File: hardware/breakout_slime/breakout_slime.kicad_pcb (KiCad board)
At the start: 2 copper layers, 54.6 x 35.6 mm, 11 parts, among them J1 Battery_Connector, J2 IMU_Conn_Female, SW1 SW_SPDT, U1 TP4056_Breakout, U2 WeMos_D1_mini, U3 BNO/MPU_Break

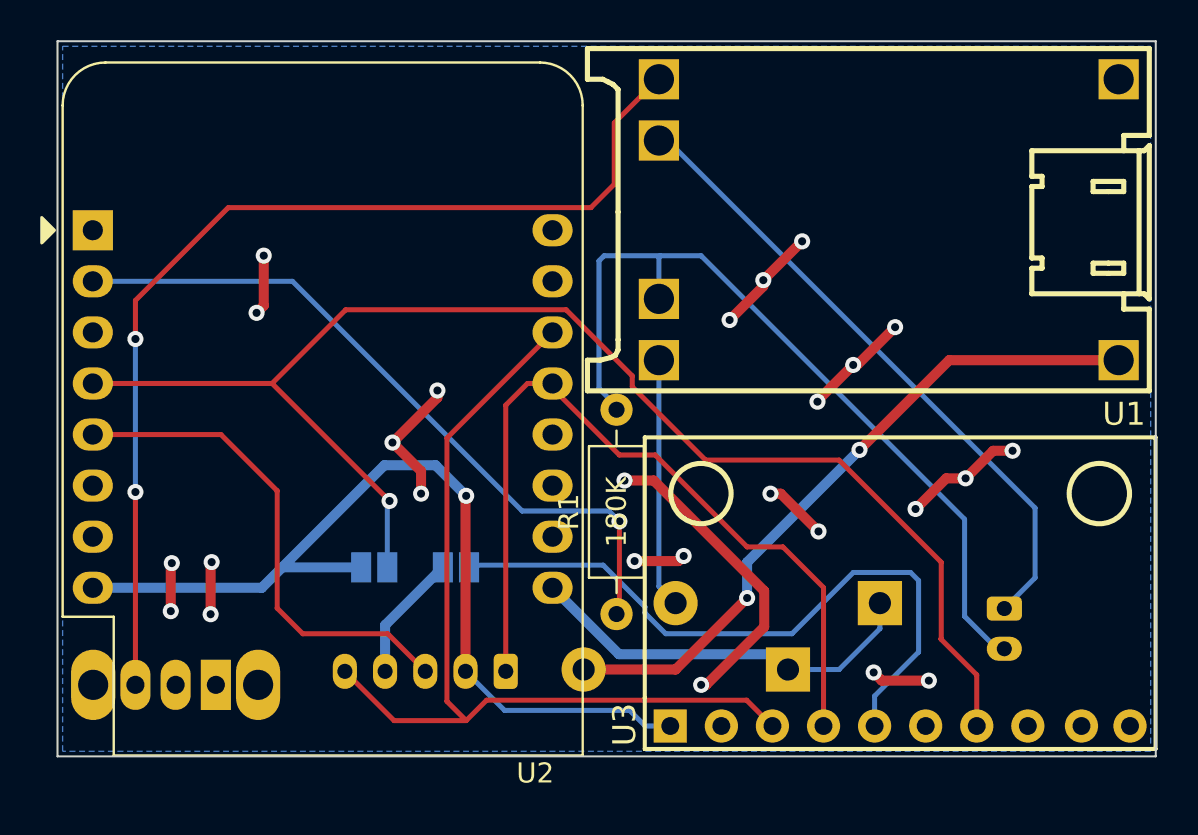
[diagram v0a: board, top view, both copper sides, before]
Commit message: breakout_slime v0.1.2
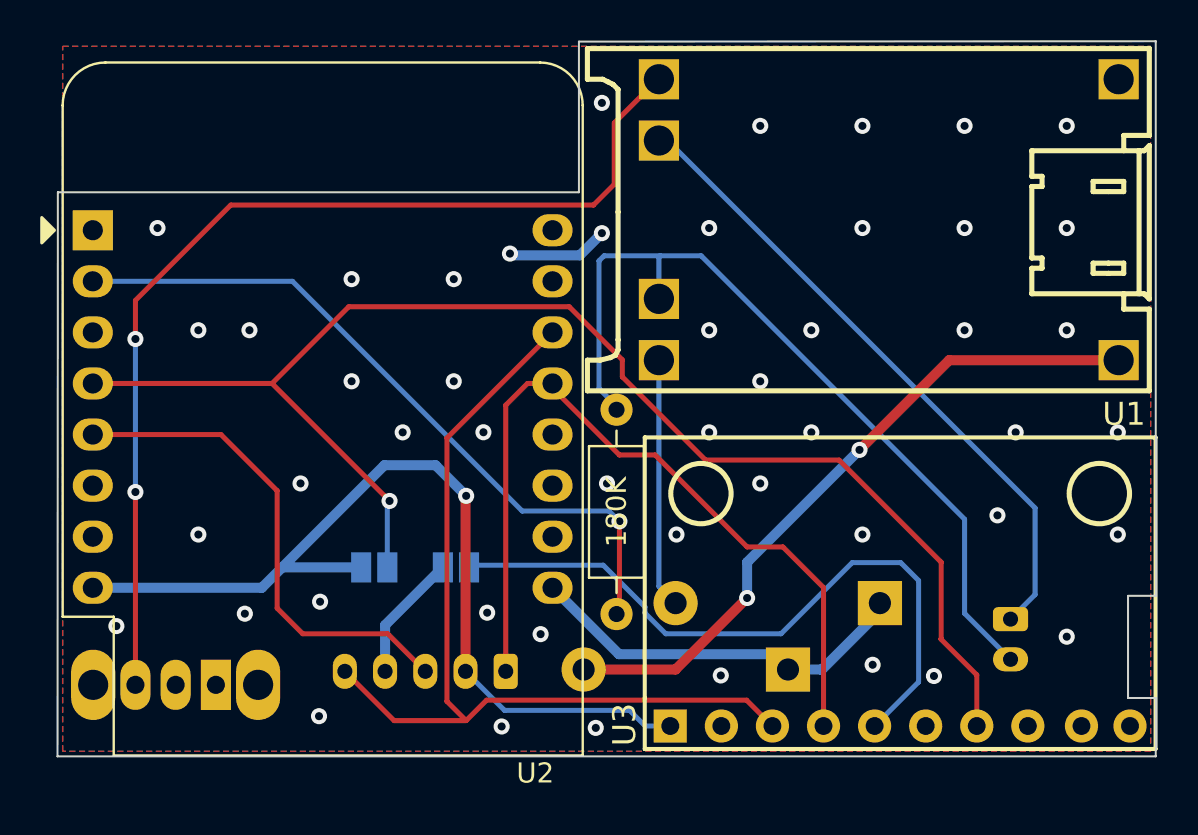
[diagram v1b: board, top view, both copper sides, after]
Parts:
- moved J1 0.61 mm to (96.3, 57.5)
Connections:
- net /5V renamed +5V
- net /B+ renamed B+
- net /INT1 renamed INT1
- net /INT2 renamed INT2
- net /SCL renamed SCL
- net /SDA renamed SDA
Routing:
- net GND: track 61.8 -> 11.4 mm, vias 26 -> 49
- net B+: track 40.8 -> 41.6 mm
- added copper zone on F.Cu, net GND
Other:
- outline, holes or cut-outs redrawn
- board text added: "${REVISION}"
